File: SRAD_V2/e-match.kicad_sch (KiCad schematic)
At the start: 28 parts, among them IC1 NCV81071BZR2G, IC2 NCV81071BZR2G, J2 691210910002, J3 691210910002, J4 691210910002, J5 691210910002, Q1 FDS6630A, Q2 FDS6630A, Q3 RQ6E080AJ, Q4 RQ6E080AJ, U3 TMCS1108A2UQDR

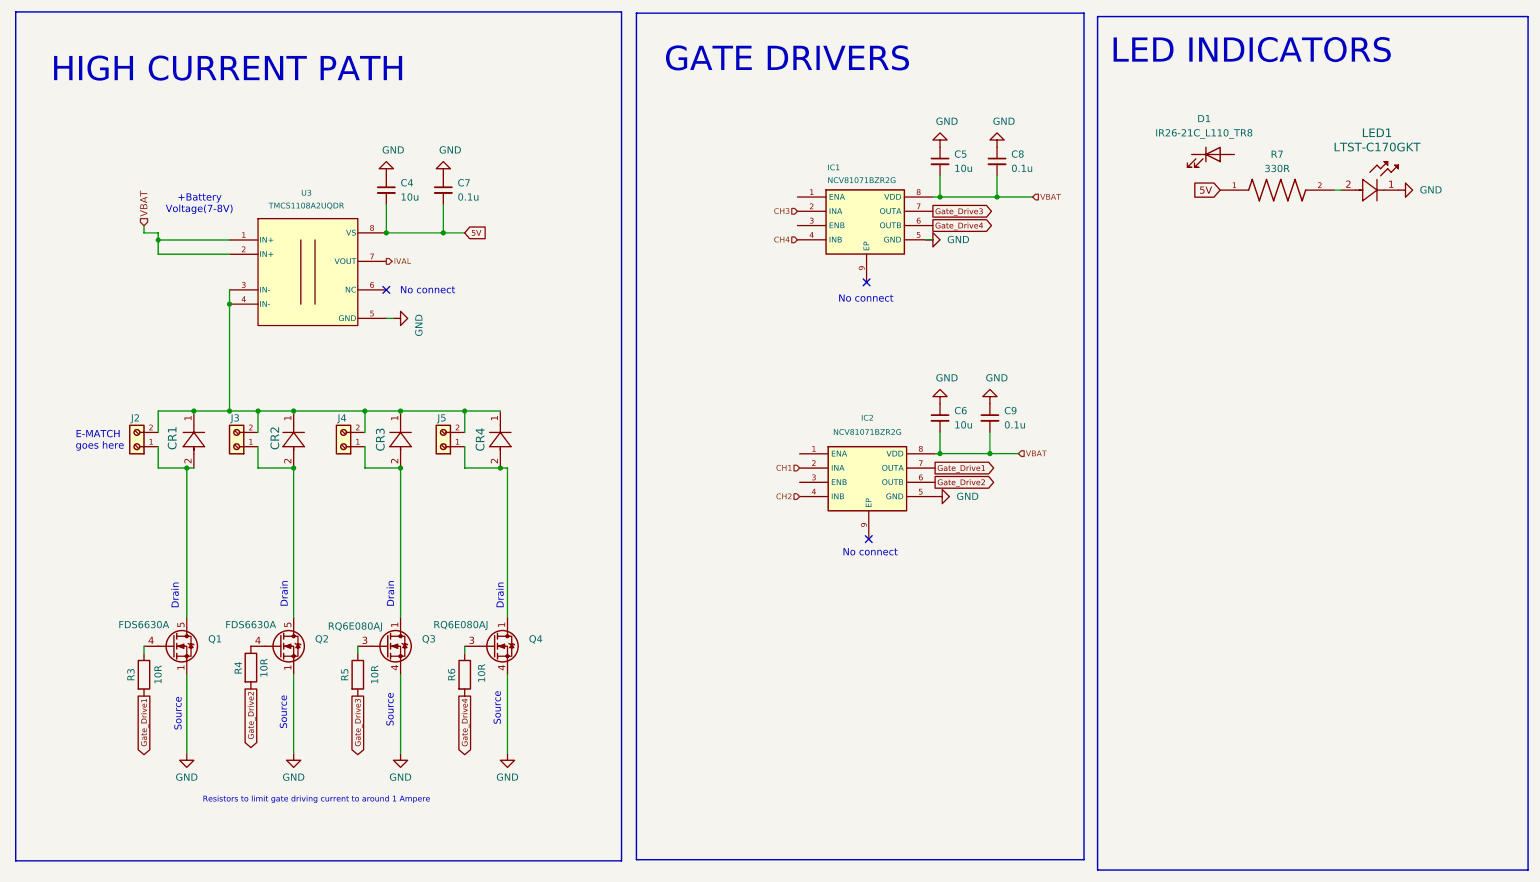
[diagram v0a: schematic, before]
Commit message: PDS routing
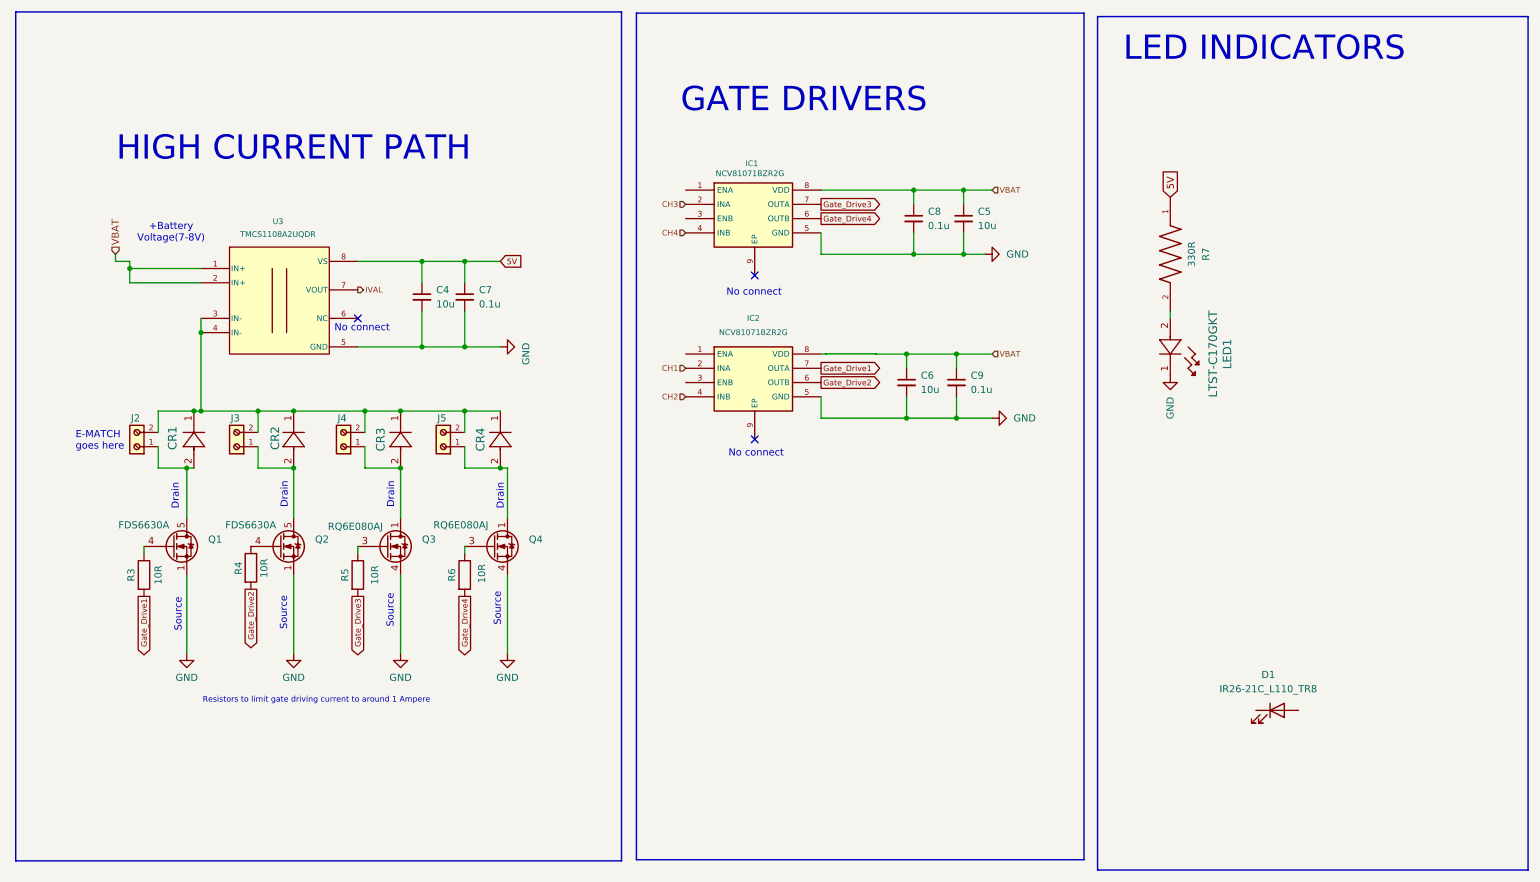
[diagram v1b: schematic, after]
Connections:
- net 5V: now also C4.1, C7.1; no longer C4.2, C7.2
- net GND: now also C4.2, C5.2, C6.2, C7.2, C8.2, C9.2; no longer C4.1, C5.1, C6.1, C7.1, C8.1, C9.1
- net VBAT: now also C5.1, C6.1, C8.1, C9.1; no longer C5.2, C6.2, C8.2, C9.2
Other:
- moved on the sheet: C4, C5, C6, C7, C8, C9, D1, IC1, IC2, LED1, Q1, Q2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
